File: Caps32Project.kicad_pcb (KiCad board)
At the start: 2 copper layers, 28 x 28 mm, 26 parts, among them J1 Ph 2.0, J2 Sh 1.0, P1 USB_C_Plug_USB2.0, Q1 AO3401A, U1 MPU-6050, U2 MAX17048G_T10, U3 ESP32C3_SuperMini, U4 MCP73831-2-OT

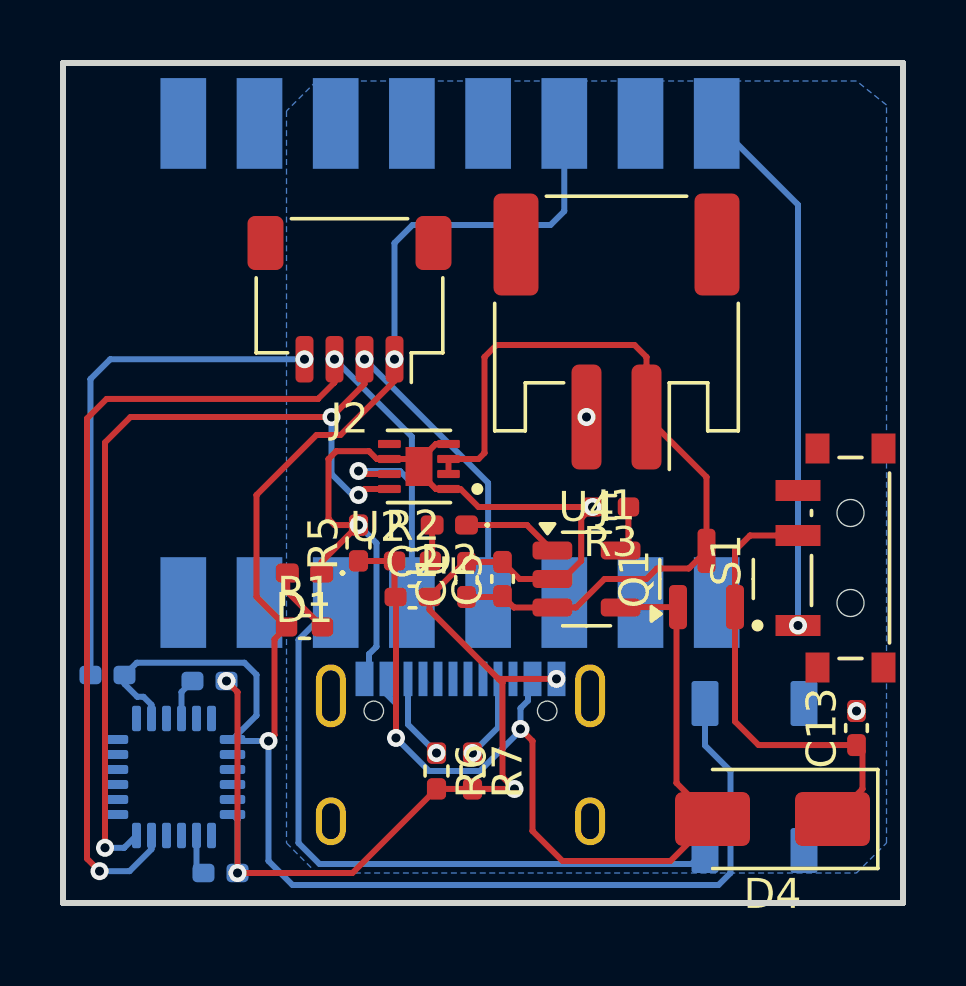
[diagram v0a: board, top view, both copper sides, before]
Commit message: Update Caps32Project.kicad_pcb
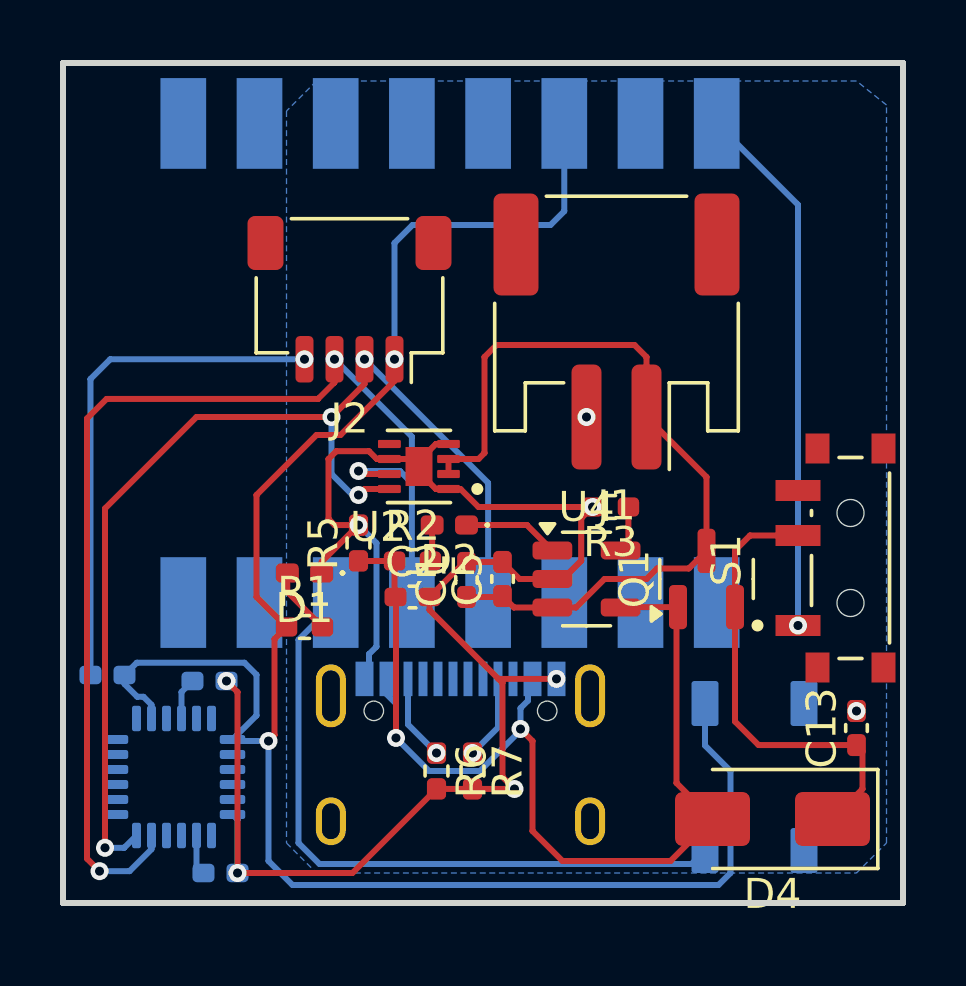
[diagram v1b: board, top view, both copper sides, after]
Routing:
- net SDA: track 39.0 -> 37.7 mm
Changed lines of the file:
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@@
-	)
-	(segment
-		(start 26.95 38.05)
-		(end 26.95 51.559998)
-		(width 0.2)
-		(layer "F.Cu")
-		(net 1)
-	)
-	(segment
-		(start 34.5 37.2)
-		(end 27.8 37.2)
-		(width 0.2)
-		(layer "F.Cu")
-		(net 1)
 	)
 	(segment
@@
 	)
 	(segment
+		(start 26.95 40.25)
+		(end 26.95 51.559998)
+		(width 0.2)
+		(layer "F.Cu")
+		(net 1)
+	)
+	(segment
+		(start 34.5 37.2)
+		(end 30 37.2)
+		(width 0.2)
+		(layer "F.Cu")
+		(net 1)
+	)
+	(segment
 		(start 35.6 36.1)
 		(end 34.5 37.2)
@@
 	)
 	(segment
-		(start 27.8 37.2)
-		(end 26.95 38.05)
+		(start 30 37.2)
+		(end 26.95 40.25)
 		(width 0.2)
 		(layer "F.Cu")

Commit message: Update Caps32Project.kicad_pcb
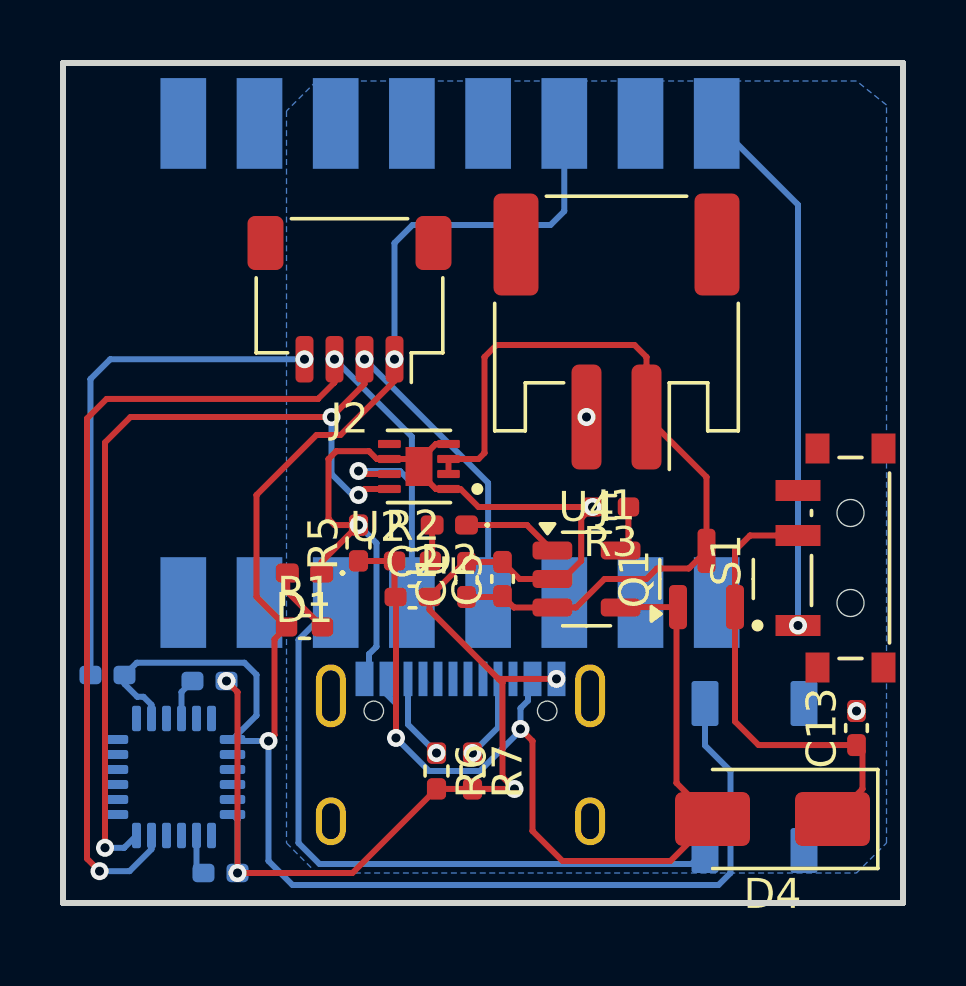
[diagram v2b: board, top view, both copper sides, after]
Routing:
- net SDA: track 37.7 -> 39.0 mm
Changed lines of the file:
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@@
+	)
+	(segment
+		(start 26.95 38.05)
+		(end 26.95 51.559998)
+		(width 0.2)
+		(layer "F.Cu")
+		(net 1)
+	)
+	(segment
+		(start 34.5 37.2)
+		(end 27.8 37.2)
+		(width 0.2)
+		(layer "F.Cu")
+		(net 1)
 	)
 	(segment
@@
 	)
 	(segment
-		(start 26.95 40.25)
-		(end 26.95 51.559998)
-		(width 0.2)
-		(layer "F.Cu")
-		(net 1)
-	)
-	(segment
-		(start 34.5 37.2)
-		(end 30 37.2)
+		(start 27.8 37.2)
+		(end 26.95 38.05)
 		(width 0.2)
 		(layer "F.Cu")
@@
 		(width 0.2)
 		(layer "F.Cu")
-		(net 1)
-	)
-	(segment
-		(start 30 37.2)
-		(end 26.95 40.25)
-		(width 0.2)
-		(layer "F.Cu")

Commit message: Update Board
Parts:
- removed C1, C13, C6: 1.0uF, Capacitor_SMD:C_0402_1005Metric_Pad0.74x0.62mm_HandSolder
- removed C2, C5: 4.7uF, Capacitor_SMD:C_0402_1005Metric_Pad0.74x0.62mm_HandSolder
- removed C3: 2.2nF, Capacitor_SMD:C_0402_1005Metric_Pad0.74x0.62mm_HandSolder
- removed C4: 0.1uF, Capacitor_SMD:C_0402_1005Metric_Pad0.74x0.62mm_HandSolder
- removed D1, D2: LED, LED_SMD:LED_0402_1005Metric_Pad0.77x0.64mm_HandSolder
- removed D3: WS2812B, LED_SMD:LED_WS2812B_PLCC4_5.0x5.0mm_P3.2mm
- removed D4: SS34, Diode_SMD:D_SMA
- removed J1: Ph 2.0, Connector_JST:JST_PH_S2B-PH-SM4-TB_1x02-1MP_P2.00mm_Horizontal
- removed J2: Sh 1.0, Connector_JST:JST_SH_SM04B-SRSS-TB_1x04-1MP_P1.00mm_Horizontal
- removed P1: USB_C_Plug_USB2.0, Connector_USB:USB_C_Receptacle_XKB_U262-16XN-4BVC11
- removed Q1: AO3401A, Package_TO_SOT_SMD:SOT-23
- removed R1, R2: 1K, Resistor_SMD:R_0402_1005Metric_Pad0.72x0.64mm_HandSolder
- removed R3: 2K, Resistor_SMD:R_0402_1005Metric_Pad0.72x0.64mm_HandSolder
- removed R5: 10K, Resistor_SMD:R_0402_1005Metric_Pad0.72x0.64mm_HandSolder
- removed R6, R7: 5.1K, Resistor_SMD:R_0402_1005Metric_Pad0.72x0.64mm_HandSolder
- removed S1: SSSS811101, Custom:SW_SSSS811101
- removed U1: MPU-6050, Sensor_Motion:InvenSense_QFN-24_4x4mm_P0.5mm
- removed U2: MAX17048G_T10, Custom:SON50P200X200X80-9N
- removed U3: ESP32C3_SuperMini, Custom:ESP32C3_Supermini_SMD
- removed U4: MCP73831-2-OT, Package_TO_SOT_SMD:SOT-23-5
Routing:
- net GND: track 75.6 -> 0.00 mm, vias 9 -> 0
- net +3V3: track 65.0 -> 0.00 mm, vias 2 -> 0
- net SCL: track 39.5 -> 0.00 mm, vias 3 -> 0
- net SDA: track 39.0 -> 0.00 mm, vias 4 -> 0
- net VBUS: track 36.3 -> 0.00 mm, vias 2 -> 0
- net +BATT: track 27.0 -> 0.00 mm
- net RGB: track 22.6 -> 0.00 mm
- net Net-(S1-Pad1): track 17.9 -> 0.00 mm, vias 1 -> 0
- net +5V: track 15.3 -> 0.00 mm
- net Net-(D2-K): track 3.21 -> 0.00 mm
- net Net-(P1-CC2): track 2.86 -> 0.00 mm, vias 1 -> 0
- net Net-(P1-CC1): track 2.82 -> 0.00 mm, vias 1 -> 0
- net Net-(D1-A): track 2.28 -> 0.00 mm
- net Net-(U4-PROG): track 1.56 -> 0.00 mm
- net Net-(U1-REGOUT): track 1.40 -> 0.00 mm
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- removed copper zone on B.Cu, net GND
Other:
- board outline removed
